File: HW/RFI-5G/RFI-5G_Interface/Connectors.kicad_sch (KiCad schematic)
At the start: 5 parts, among them J1 Conn_01x10_Female, J2 Conn_01x10_Female, J3 Conn_01x10_Female, J4 Conn_01x10_Female, J5 Conn_01x04_Female

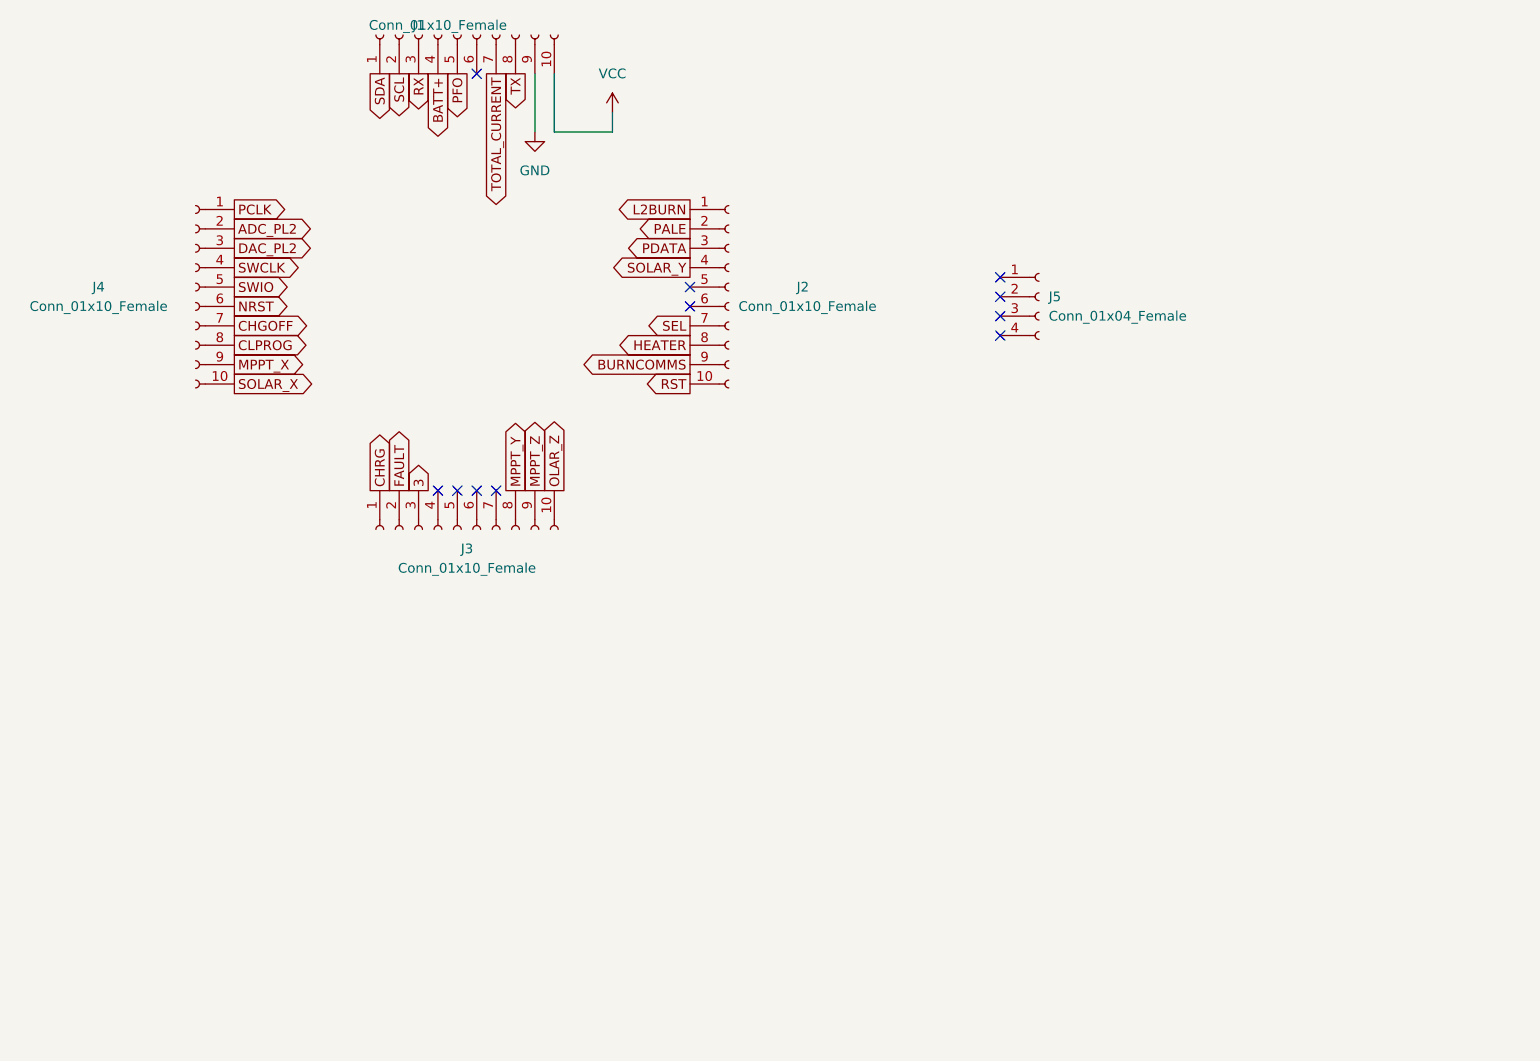
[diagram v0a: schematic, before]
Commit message: RF top and Bottom boards
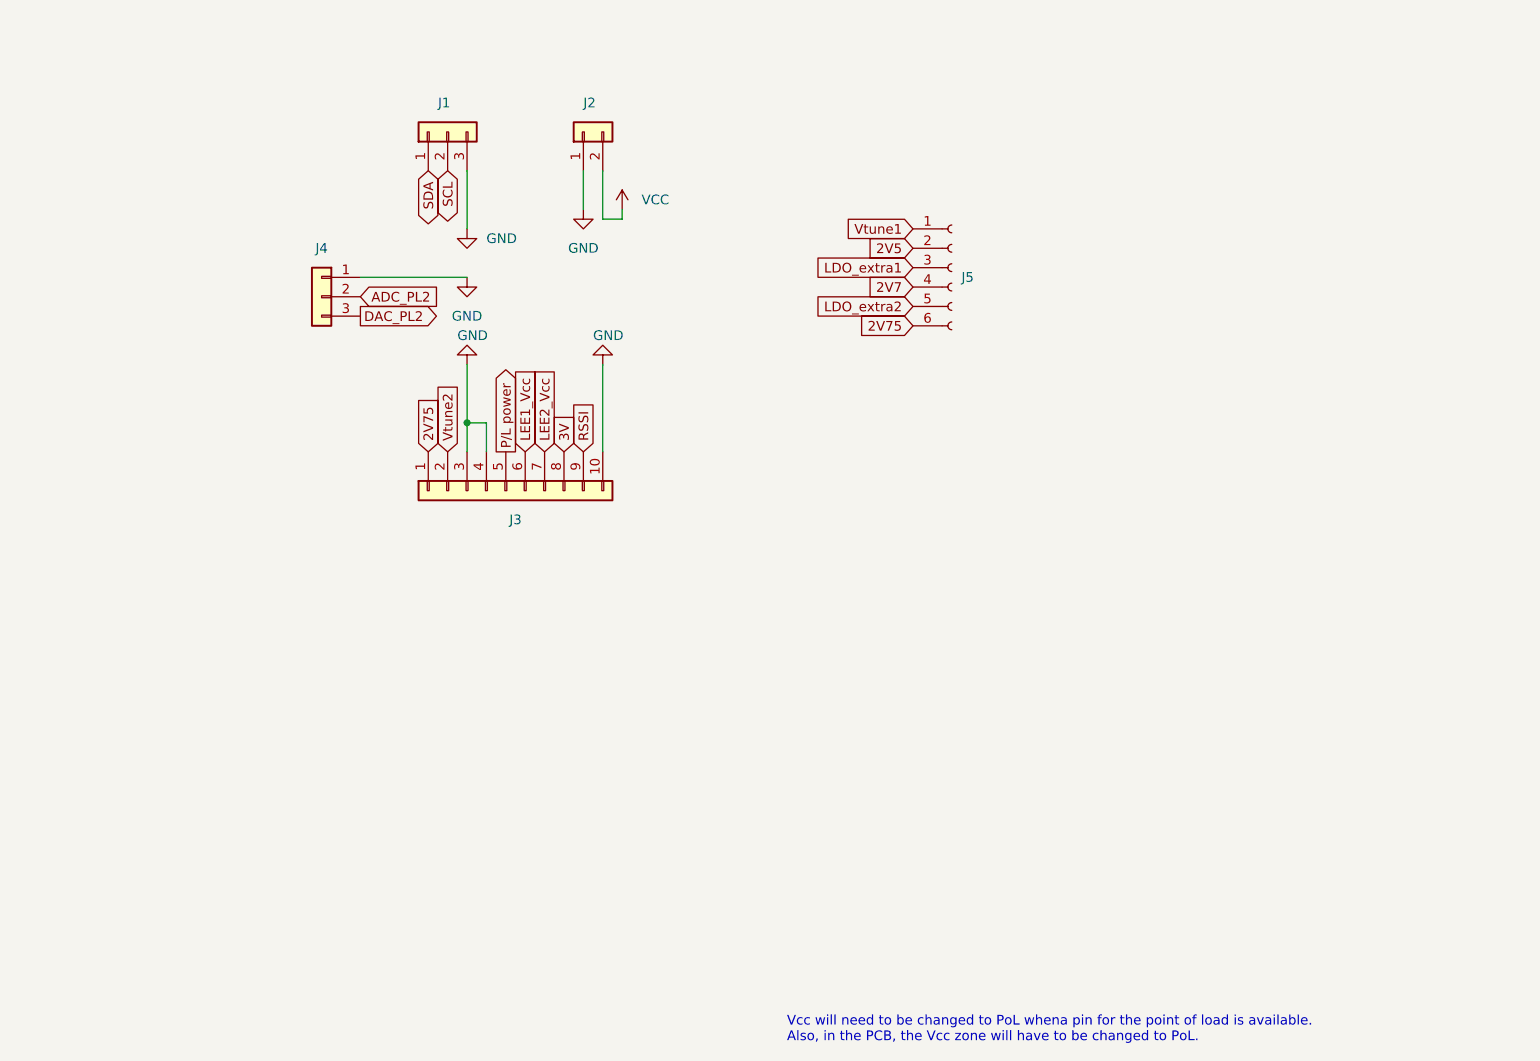
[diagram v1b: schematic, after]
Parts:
- removed J1, J2, J3, J4: Conn_01x10_Female, Connector_PinHeader_2.54mm:PinHeader_1x10_P2.54mm_Vertical, symbol Connector:Conn_01x10_Female
- removed J5: Conn_01x04_Female, Connector_PinHeader_2.54mm:PinHeader_1x04_P2.54mm_Vertical, symbol Connector:Conn_01x04_Female
- added J1, J4: Conn_01x03, Connector_PinHeader_2.54mm:PinHeader_1x03_P2.54mm_Vertical, symbol Connector_Generic:Conn_01x03
- added J2: Conn_01x02, Connector_PinHeader_2.54mm:PinHeader_1x02_P2.54mm_Vertical, symbol Connector_Generic:Conn_01x02
- added J3: Conn_01x10, Connector_PinHeader_2.54mm:PinHeader_1x10_P2.54mm_Vertical, symbol Connector_Generic:Conn_01x10
- added J5: Conn_01x06_Female, Connector_PinHeader_1.00mm:PinHeader_1x06_P1.00mm_Vertical, symbol Connector:Conn_01x06_Female
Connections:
- net ADC_PL2: now also J4.2 (Pin_2)
- net DAC_PL2: now also J4.3 (Pin_3)
- net GND: now also J1.3 (Pin_3), J2.1 (Pin_1), J3.10 (Pin_10), J3.3 (Pin_3), J3.4 (Pin_4), J4.1 (Pin_1)
- net SCL: now also J1.2 (Pin_2)
- net SDA: now also J1.1 (Pin_1)
- net VCC: now also J2.2 (Pin_2)
- new net 2V5: J5.2 (Pin_2)
- new net 2V7: J5.4 (Pin_4)
- new net 2V75: J3.1 (Pin_1), J5.6 (Pin_6)
- new net 3V: J3.8 (Pin_8)
- new net LDO_extra1: J5.3 (Pin_3)
- new net LDO_extra2: J5.5 (Pin_5)
- new net LEE1_Vcc: J3.6 (Pin_6)
- new net LEE2_Vcc: J3.7 (Pin_7)
- new net P/L power: J3.5 (Pin_5)
- new net RSSI: J3.9 (Pin_9)
- new net Vtune1: J5.1 (Pin_1)
- new net Vtune2: J3.2 (Pin_2)
- no-connect marks 11 -> 0
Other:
- note added: "Vcc will need to be changed to PoL whena pin for the point of load is available. Also, in the PCB, the Vcc zone will have to be changed to PoL."

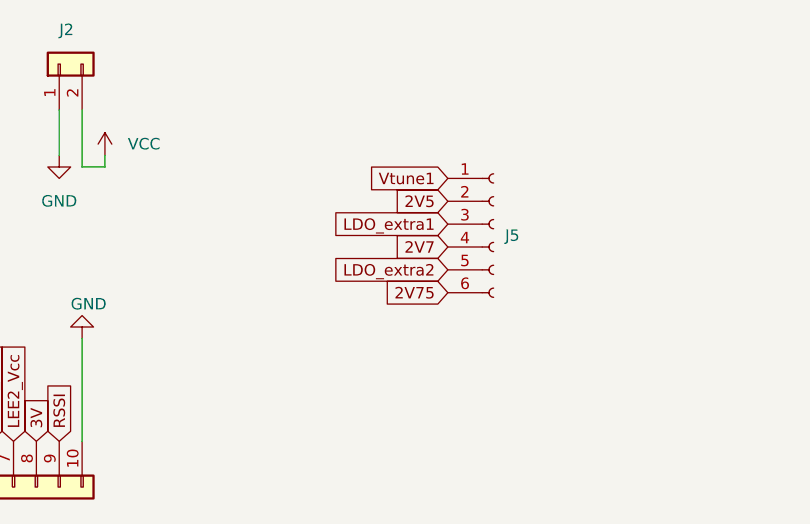
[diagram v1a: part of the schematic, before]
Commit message: PL boards
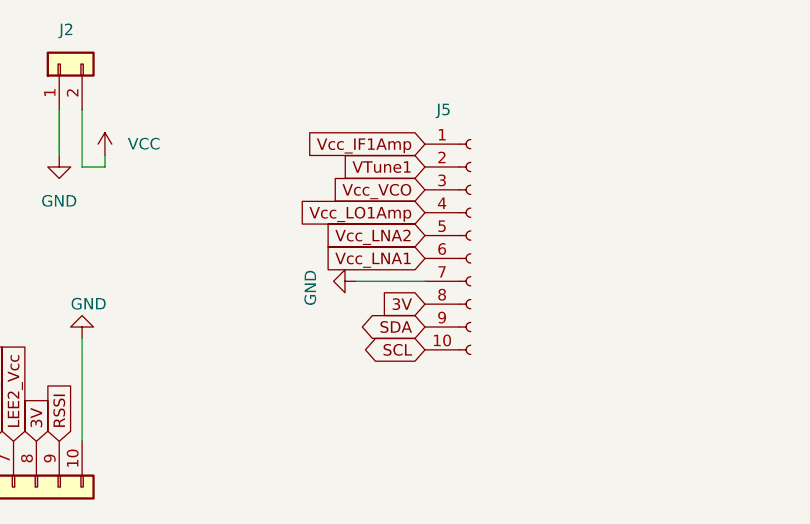
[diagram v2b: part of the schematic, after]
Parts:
- removed J5: Conn_01x06_Female, Connector_PinHeader_1.00mm:PinHeader_1x06_P1.00mm_Vertical, symbol Connector:Conn_01x06_Female
- added J5: Conn_01x10_Female, Connector_PinHeader_1.00mm:PinHeader_1x10_P1.00mm_Vertical, symbol Connector:Conn_01x10_Female
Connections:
- net 3V: now also J5.8 (Pin_8)
- net GND: now also J5.7 (Pin_7)
- net SCL: now also J5.10 (Pin_10)
- net SDA: now also J5.9 (Pin_9)
- new net VTune1: J5.2 (Pin_2)
- new net Vcc_IF1Amp: J5.1 (Pin_1)
- new net Vcc_LNA1: J5.6 (Pin_6)
- new net Vcc_LNA2: J5.5 (Pin_5)
- new net Vcc_LO1Amp: J5.4 (Pin_4)
- new net Vcc_VCO: J5.3 (Pin_3)
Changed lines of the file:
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@@
+    (stroke (width 0) (type default) (color 0 0 0 0))
+  )
+  (wire (pts (xy 184.15 76.2) (xy 191.77 76.2))
     (stroke (width 0) (type default) (color 0 0 0 0))
   )
@@
     )
   )
-  (global_label "LDO_extra1" (shape input) (at 194.31 69.85 180) (fields_autoplaced)
-    (effects (font (size 1.27 1.27)) (justify right))
-    (property "Intersheet References" "${INTERSHEET_REFS}" (id 0) (at 181.3136 69.7706 0)
-      (effects (font (size 1.27 1.27)) (justify right) hide)
-    )
-  )
   (global_label "RSSI" (shape input) (at 151.13 93.98 90) (fields_autoplaced)
     (effects (font (size 1.27 1.27)) (justify left))
@@
     )
   )
-  (global_label "Vtune1" (shape input) (at 194.31 64.77 180) (fields_autoplaced)
-    (effects (font (size 1.27 1.27)) (justify right))
-    (property "Intersheet References" "${INTERSHEET_REFS}" (id 0) (at 185.4864 64.6906 0)
-      (effects (font (size 1.27 1.27)) (justify right) hide)
-    )
-  )
   (global_label "SCL" (shape bidirectional) (at 133.35 57.15 270) (fields_autoplaced)
     (effects (font (size 1.27 1.27)) (justify right))
@@
     )
   )
+  (global_label "SDA" (shape bidirectional) (at 191.77 81.28 180) (fields_autoplaced)
+    (effects (font (size 1.27 1.27)) (justify right))
+    (property "Intersheet References" "${INTERSHEET_REFS}" (id 0) (at 185.7888 81.2006 0)
+      (effects (font (size 1.27 1.27)) (justify right) hide)
+    )
+  )
   (global_label "LEE2_Vcc" (shape input) (at 146.05 93.98 90) (fields_autoplaced)
     (effects (font (size 1.27 1.27)) (justify left))
@@
     )
   )
-  (global_label "2V7" (shape input) (at 194.31 72.39 180) (fields_autoplaced)
-    (effects (font (size 1.27 1.27)) (justify right))
-    (property "Intersheet References" "${INTERSHEET_REFS}" (id 0) (at 188.3893 72.3106 0)
+  (global_label "Vcc_LNA1" (shape input) (at 191.77 73.66 180) (fields_autoplaced)
+    (effects (font (size 1.27 1.27)) (justify right))
+    (property "Intersheet References" "${INTERSHEET_REFS}" (id 0) (at 180.4669 73.5806 0)
       (effects (font (size 1.27 1.27)) (justify right) hide)
     )
@@
     )
   )
-  (global_label "2V75" (shape input) (at 194.31 77.47 180) (fields_autoplaced)
-    (effects (font (size 1.27 1.27)) (justify right))
-    (property "Intersheet References" "${INTERSHEET_REFS}" (id 0) (at 187.1798 77.3906 0)
+  (global_label "3V" (shape input) (at 191.77 78.74 180) (fields_autoplaced)
+    (effects (font (size 1.27 1.27)) (justify right))
+    (property "Intersheet References" "${INTERSHEET_REFS}" (id 0) (at 187.0588 78.6606 0)
       (effects (font (size 1.27 1.27)) (justify right) hide)
     )
@@
     )
   )
-  (global_label "2V5" (shape input) (at 194.31 67.31 180) (fields_autoplaced)
-    (effects (font (size 1.27 1.27)) (justify right))
-    (property "Intersheet References" "${INTERSHEET_REFS}" (id 0) (at 188.3893 67.2306 0)
+  (global_label "SCL" (shape bidirectional) (at 191.77 83.82 180) (fields_autoplaced)
+    (effects (font (size 1.27 1.27)) (justify right))
+    (property "Intersheet References" "${INTERSHEET_REFS}" (id 0) (at 185.8493 83.7406 0)
+      (effects (font (size 1.27 1.27)) (justify right) hide)
+    )
+  )
+  (global_label "Vcc_LNA2" (shape input) (at 191.77 71.12 180) (fields_autoplaced)
+    (effects (font (size 1.27 1.27)) (justify right))
+    (property "Intersheet References" "${INTERSHEET_REFS}" (id 0) (at 180.4669 71.0406 0)
       (effects (font (size 1.27 1.27)) (justify right) hide)
     )
@@
     )
   )
-  (global_label "LDO_extra2" (shape input) (at 194.31 74.93 180) (fields_autoplaced)
-    (effects (font (size 1.27 1.27)) (justify right))
-    (property "Intersheet References" "${INTERSHEET_REFS}" (id 0) (at 181.3136 74.8506 0)
+  (global_label "Vcc_IF1Amp" (shape input) (at 191.77 60.96 180) (fields_autoplaced)
+    (effects (font (size 1.27 1.27)) (justify right))
+    (property "Intersheet References" "${INTERSHEET_REFS}" (id 0) (at 178.2898 60.8806 0)
+      (effects (font (size 1.27 1.27)) (justify right) hide)
+    )
+  )
+  (global_label "Vcc_LO1Amp" (shape input) (at 191.77 68.58 180) (fields_autoplaced)
+    (effects (font (size 1.27 1.27)) (justify right))
+    (property "Intersheet References" "${INTERSHEET_REFS}" (id 0) (at 177.6245 68.5006 0)
+      (effects (font (size 1.27 1.27)) (justify right) hide)
+    )
+  )
+  (global_label "VTune1" (shape input) (at 191.77 63.5 180) (fields_autoplaced)
+    (effects (font (size 1.27 1.27)) (justify right))
+    (property "Intersheet References" "${INTERSHEET_REFS}" (id 0) (at 182.7045 63.4206 0)
+      (effects (font (size 1.27 1.27)) (justify right) hide)
+    )
+  )
+  (global_label "Vcc_VCO" (shape input) (at 191.77 66.04 180) (fields_autoplaced)
+    (effects (font (size 1.27 1.27)) (justify right))
+    (property "Intersheet References" "${INTERSHEET_REFS}" (id 0) (at 181.4345 65.9606 0)
       (effects (font (size 1.27 1.27)) (justify right) hide)
     )
@@
     (pin "3")
   )
-  (symbol (lib_id "Connector:Conn_01x06_Female") (at 199.39 69.85 0) (unit 1)
+  (symbol (lib_id "power:GND") (at 184.15 76.2 270) (unit 1)
+    (in_bom yes) (on_board yes)
+    (property "Reference" "#PWR?" (id 0) (at 177.8 76.2 0)
+      (effects (font (size 1.27 1.27)) hide)
+    )
+    (property "Value" "GND" (id 1) (at 179.07 74.93 0)
+      (effects (font (size 1.27 1.27)) (justify left))
+    )
+    (property "Footprint" "" (id 2) (at 184.15 76.2 0)
+      (effects (font (size 1.27 1.27)) hide)
+    )
+    (property "Datasheet" "" (id 3) (at 184.15 76.2 0)
+      (effects (font (size 1.27 1.27)) hide)
+    )
+    (pin "1")
+  )
+  (symbol (lib_id "power:VCC") (at 156.21 62.23 0) (unit 1)
     (in_bom yes) (on_board yes) (fields_autoplaced)
-    (property "Reference" "J5" (id 0) (at 200.66 71.1199 0)
+    (property "Reference" "#PWR0117" (id 0) (at 156.21 66.04 0)
+      (effects (font (size 1.27 1.27)) hide)
+    )
+    (property "Value" "VCC" (id 1) (at 158.75 60.9599 0)
       (effects (font (size 1.27 1.27)) (justify left))
     )
-    (property "Value" "Conn_01x06_Female" (id 1) (at 200.66 72.3899 0)
-      (effects (font (size 1.27 1.27)) (justify left) hide)
-    )
-    (property "Footprint" "Connector_PinHeader_1.00mm:PinHeader_1x06_P1.00mm_Vertical" (id 2) (at 199.39 69.85 0)
-      (effects (font (size 1.27 1.27)) hide)
-    )
-    (property "Datasheet" "~" (id 3) (at 199.39 69.85 0)
-      (effects (font (size 1.27 1.27)) hide)
-    )
-    (pin "1")
+    (property "Footprint" "" (id 2) (at 156.21 62.23 0)
+      (effects (font (size 1.27 1.27)) hide)
+    )
+    (property "Datasheet" "" (id 3) (at 156.21 62.23 0)
+      (effects (font (size 1.27 1.27)) hide)
+    )
+    (pin "1")
+  )
+  (symbol (lib_id "power:GND") (at 151.13 62.23 0) (unit 1)
+    (in_bom yes) (on_board yes) (fields_autoplaced)
+    (property "Reference" "#PWR0103" (id 0) (at 151.13 68.58 0)
+      (effects (font (size 1.27 1.27)) hide)
+    )
+    (property "Value" "GND" (id 1) (at 151.13 67.31 0))
+    (property "Footprint" "" (id 2) (at 151.13 62.23 0)
+      (effects (font (size 1.27 1.27)) hide)
+    )
+    (property "Datasheet" "" (id 3) (at 151.13 62.23 0)
+      (effects (font (size 1.27 1.27)) hide)
+    )
+    (pin "1")
+  )
+  (symbol (lib_id "Connector:Conn_01x10_Female") (at 196.85 71.12 0) (unit 1)
+    (in_bom yes) (on_board yes)
+    (property "Reference" "J5" (id 0) (at 193.04 57.15 0)
+      (effects (font (size 1.27 1.27)) (justify left))
+    )
+    (property "Value" "Conn_01x10_Female" (id 1) (at 198.12 73.6599 0)
+      (effects (font (size 1.27 1.27)) (justify left) hide)
+    )
+    (property "Footprint" "Connector_PinHeader_1.00mm:PinHeader_1x10_P1.00mm_Vertical" (id 2) (at 196.85 71.12 0)
+      (effects (font (size 1.27 1.27)) hide)
+    )
+    (property "Datasheet" "~" (id 3) (at 196.85 71.12 0)
+      (effects (font (size 1.27 1.27)) hide)
+    )
+    (pin "1")
+    (pin "10")
     (pin "2")
     (pin "3")
@@
     (pin "5")
     (pin "6")
-  )
-  (symbol (lib_id "power:VCC") (at 156.21 62.23 0) (unit 1)
-    (in_bom yes) (on_board yes) (fields_autoplaced)
-    (property "Reference" "#PWR0117" (id 0) (at 156.21 66.04 0)
-      (effects (font (size 1.27 1.27)) hide)
-    )
-    (property "Value" "VCC" (id 1) (at 158.75 60.9599 0)
-      (effects (font (size 1.27 1.27)) (justify left))
-    )
-    (property "Footprint" "" (id 2) (at 156.21 62.23 0)
-      (effects (font (size 1.27 1.27)) hide)
-    )
-    (property "Datasheet" "" (id 3) (at 156.21 62.23 0)
-      (effects (font (size 1.27 1.27)) hide)
-    )
-    (pin "1")
-  )
-  (symbol (lib_id "power:GND") (at 151.13 62.23 0) (unit 1)
-    (in_bom yes) (on_board yes) (fields_autoplaced)
-    (property "Reference" "#PWR0103" (id 0) (at 151.13 68.58 0)
-      (effects (font (size 1.27 1.27)) hide)
-    )
-    (property "Value" "GND" (id 1) (at 151.13 67.31 0))
-    (property "Footprint" "" (id 2) (at 151.13 62.23 0)
-      (effects (font (size 1.27 1.27)) hide)
-    )
-    (property "Datasheet" "" (id 3) (at 151.13 62.23 0)
-      (effects (font (size 1.27 1.27)) hide)
-    )
-    (pin "1")
+    (pin "7")
+    (pin "8")
+    (pin "9")
   )
   (symbol (lib_id "Connector_Generic:Conn_01x10") (at 140.97 99.06 90) (mirror x) (unit 1)
